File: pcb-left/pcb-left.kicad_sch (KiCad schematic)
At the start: 39 parts, among them J3 BAT, U1 xiao-ble

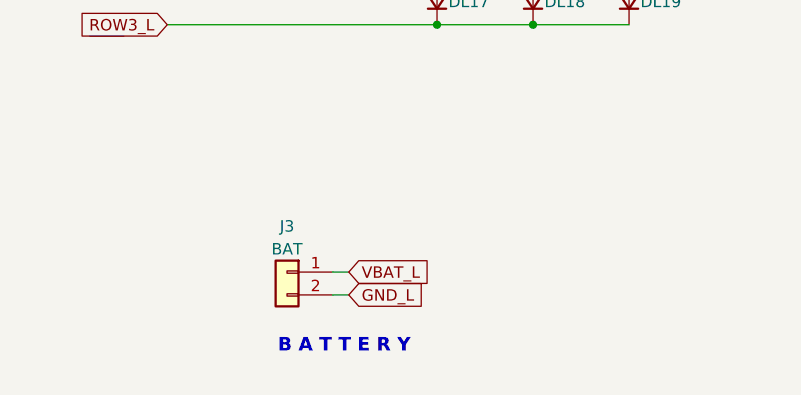
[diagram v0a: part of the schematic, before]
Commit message: Update schematic and pcb to rev 0.32
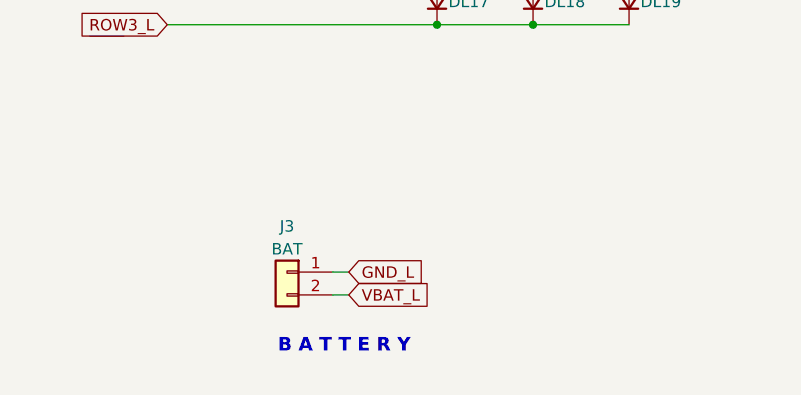
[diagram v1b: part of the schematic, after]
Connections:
- net GND_L: now also J3.1 (Pin_1); no longer J3.2 (Pin_2)
- net VBAT_L: now also J3.2 (Pin_2); no longer J3.1 (Pin_1)
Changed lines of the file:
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@@
     (title "Karma Wireless Split Ergonomic Keyboard")
     (date "2023-04-04")
-    (rev "0.3")
+    (rev "0.32")
   )
   (junction (at 70.358 51.689) (diameter 0) (color 0 0 0 0)
@@
     )
   )
-  (global_label "VBAT_L" (shape input) (at 54.9656 134.2898 0) (fields_autoplaced)
+  (global_label "GND_L" (shape input) (at 54.9656 134.2898 0) (fields_autoplaced)
     (effects (font (size 1.27 1.27)) (justify left))
-    (property "Intersheetrefs" "${INTERSHEET_REFS}" (at 64.2819 134.2898 0)
+    (property "Intersheetrefs" "${INTERSHEET_REFS}" (at 63.7376 134.2898 0)
       (effects (font (size 1.27 1.27)) (justify left) hide)
     )
@@
     )
   )
-  (global_label "GND_L" (shape input) (at 54.9656 136.8298 0) (fields_autoplaced)
+  (global_label "VBAT_L" (shape input) (at 54.9656 136.8298 0) (fields_autoplaced)
     (effects (font (size 1.27 1.27)) (justify left))
-    (property "Intersheetrefs" "${INTERSHEET_REFS}" (at 63.2449 136.7504 0)
+    (property "Intersheetrefs" "${INTERSHEET_REFS}" (at 64.2819 136.8298 0)
       (effects (font (size 1.27 1.27)) (justify left) hide)
     )
@@
         )
       )
-      (project "left-pcb"
+      (project "pcb-left"
         (path "/f98b87e5-a6a7-4c83-9bb9-aca334f9bfc8"
           (reference "SWL16") (unit 1)
@@
         )
       )
-      (project "left-pcb"
+      (project "pcb-left"
         (path "/f98b87e5-a6a7-4c83-9bb9-aca334f9bfc8"
           (reference "J1") (unit 1)
@@
         )
       )
-      (project "left-pcb"
+      (project "pcb-left"
         (path "/f98b87e5-a6a7-4c83-9bb9-aca334f9bfc8"
           (reference "SWL9") (unit 1)
@@
         )
       )
-      (project "left-pcb"
+      (project "pcb-left"
         (path "/f98b87e5-a6a7-4c83-9bb9-aca334f9bfc8"
           (reference "DL18") (unit 1)
@@
         )
       )
-      (project "left-pcb"
+      (project "pcb-left"
         (path "/f98b87e5-a6a7-4c83-9bb9-aca334f9bfc8"
           (reference "DL6") (unit 1)
@@
         )
       )
-      (project "left-pcb"
+      (project "pcb-left"
         (path "/f98b87e5-a6a7-4c83-9bb9-aca334f9bfc8"
           (reference "DL9") (unit 1)
@@
         )
       )
-      (project "left-pcb"
+      (project "pcb-left"
         (path "/f98b87e5-a6a7-4c83-9bb9-aca334f9bfc8"
           (reference "RSW1") (unit 1)
@@
         )
       )
-      (project "left-pcb"
+      (project "pcb-left"
         (path "/f98b87e5-a6a7-4c83-9bb9-aca334f9bfc8"
           (reference "SWL5") (unit 1)
@@
         )
       )
-      (project "left-pcb"
+      (project "pcb-left"
         (path "/f98b87e5-a6a7-4c83-9bb9-aca334f9bfc8"
           (reference "SWL7") (unit 1)
@@
         )
       )
-      (project "left-pcb"
+      (project "pcb-left"
         (path "/f98b87e5-a6a7-4c83-9bb9-aca334f9bfc8"
           (reference "SWL11") (unit 1)
@@
         )
       )
-      (project "left-pcb"
+      (project "pcb-left"
         (path "/f98b87e5-a6a7-4c83-9bb9-aca334f9bfc8"
           (reference "DL15") (unit 1)
@@
         )
       )
-      (project "left-pcb"
+      (project "pcb-left"
         (path "/f98b87e5-a6a7-4c83-9bb9-aca334f9bfc8"
           (reference "SWL10") (unit 1)
@@
         )
       )
-      (project "left-pcb"
+      (project "pcb-left"
         (path "/f98b87e5-a6a7-4c83-9bb9-aca334f9bfc8"
           (reference "SWL3") (unit 1)
@@
         )
       )
-      (project "left-pcb"
+      (project "pcb-left"
         (path "/f98b87e5-a6a7-4c83-9bb9-aca334f9bfc8"
           (reference "SWL14") (unit 1)
@@
         )
       )
-      (project "left-pcb"
+      (project "pcb-left"
         (path "/f98b87e5-a6a7-4c83-9bb9-aca334f9bfc8"
           (reference "DL11") (unit 1)
@@
         )
       )
-      (project "left-pcb"
+      (project "pcb-left"
         (path "/f98b87e5-a6a7-4c83-9bb9-aca334f9bfc8"
           (reference "SWL8") (unit 1)
@@
         )
       )
-      (project "left-pcb"
+      (project "pcb-left"
         (path "/f98b87e5-a6a7-4c83-9bb9-aca334f9bfc8"
           (reference "SWL13") (unit 1)
@@
         )
       )
-      (project "left-pcb"
+      (project "pcb-left"
         (path "/f98b87e5-a6a7-4c83-9bb9-aca334f9bfc8"
           (reference "DL16") (unit 1)
@@
         )
       )
-      (project "left-pcb"
+      (project "pcb-left"
         (path "/f98b87e5-a6a7-4c83-9bb9-aca334f9bfc8"
           (reference "DL8") (unit 1)
@@
         )
       )
-      (project "left-pcb"
+      (project "pcb-left"
         (path "/f98b87e5-a6a7-4c83-9bb9-aca334f9bfc8"
           (reference "DL4") (unit 1)
@@
         )
       )
-      (project "left-pcb"
+      (project "pcb-left"
         (path "/f98b87e5-a6a7-4c83-9bb9-aca334f9bfc8"
           (reference "SWL18") (unit 1)
@@
         )
       )
-      (project "left-pcb"
+      (project "pcb-left"
         (path "/f98b87e5-a6a7-4c83-9bb9-aca334f9bfc8"
           (reference "SWL6") (unit 1)
@@
         )
       )
-      (project "left-pcb"
+      (project "pcb-left"
         (path "/f98b87e5-a6a7-4c83-9bb9-aca334f9bfc8"
           (reference "SWL12") (unit 1)
@@
         )
       )
-      (project "left-pcb"
+      (project "pcb-left"
         (path "/f98b87e5-a6a7-4c83-9bb9-aca334f9bfc8"
           (reference "SWL2") (unit 1)
@@
         )
       )
-      (project "left-pcb"
+      (project "pcb-left"
         (path "/f98b87e5-a6a7-4c83-9bb9-aca334f9bfc8"
           (reference "SWL1") (unit 1)
@@
         )
       )
-      (project "left-pcb"
+      (project "pcb-left"
         (path "/f98b87e5-a6a7-4c83-9bb9-aca334f9bfc8"
           (reference "SWL4") (unit 1)
@@
         )
       )
-      (project "left-pcb"
+      (project "pcb-left"
         (path "/f98b87e5-a6a7-4c83-9bb9-aca334f9bfc8"
           (reference "DL2") (unit 1)
@@
         )
       )
-      (project "left-pcb"
+      (project "pcb-left"
         (path "/f98b87e5-a6a7-4c83-9bb9-aca334f9bfc8"
           (reference "DL3") (unit 1)
@@
         )
       )
-      (project "left-pcb"
+      (project "pcb-left"
         (path "/f98b87e5-a6a7-4c83-9bb9-aca334f9bfc8"
           (reference "U1") (unit 1)
@@
         )
       )
-      (project "left-pcb"
+      (project "pcb-left"
         (path "/f98b87e5-a6a7-4c83-9bb9-aca334f9bfc8"
           (reference "DL1") (unit 1)
@@
         )
       )
-      (project "left-pcb"
+      (project "pcb-left"
         (path "/f98b87e5-a6a7-4c83-9bb9-aca334f9bfc8"
           (reference "DL12") (unit 1)
@@
         )
       )
-      (project "left-pcb"
+      (project "pcb-left"
         (path "/f98b87e5-a6a7-4c83-9bb9-aca334f9bfc8"
           (reference "SWL17") (unit 1)
@@
         )
       )
-      (project "left-pcb"
+      (project "pcb-left"
         (path "/f98b87e5-a6a7-4c83-9bb9-aca334f9bfc8"
           (reference "DL17") (unit 1)
@@
         )
       )
-      (project "left-pcb"
+      (project "pcb-left"
         (path "/f98b87e5-a6a7-4c83-9bb9-aca334f9bfc8"
           (reference "DL7") (unit 1)
@@
         )
       )
-      (project "left-pcb"
+      (project "pcb-left"
         (path "/f98b87e5-a6a7-4c83-9bb9-aca334f9bfc8"
           (reference "DL14") (unit 1)
@@
         )
       )
-      (project "left-pcb"
+      (project "pcb-left"
         (path "/f98b87e5-a6a7-4c83-9bb9-aca334f9bfc8"
           (reference "DL10") (unit 1)
@@
         )
       )
-      (project "left-pcb"
+      (project "pcb-left"
         (path "/f98b87e5-a6a7-4c83-9bb9-aca334f9bfc8"
           (reference "DL5") (unit 1)
@@
         )
       )
-      (project "left-pcb"
+      (project "pcb-left"
         (path "/f98b87e5-a6a7-4c83-9bb9-aca334f9bfc8"
           (reference "SWL15") (unit 1)
@@
         )
       )
-      (project "left-pcb"
+      (project "pcb-left"
         (path "/f98b87e5-a6a7-4c83-9bb9-aca334f9bfc8"
           (reference "DL13") (unit 1)
